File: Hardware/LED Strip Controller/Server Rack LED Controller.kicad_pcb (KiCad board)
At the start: 2 copper layers, 134.6 x 76.2 mm, 168 parts, among them J1 LED_ONE_PWR, J10 UART, J11 CONN_2, J12 LED_THREE_PWR, J13 CONN_3, J14 LED_FOUR_PWR, J15 Conn_01x06_Male, J16 CONN_4, J17 TST, J18 Conn_01x02_Female, J19 Conn_02x04_Odd_Even, J2 Screw_Terminal_01x02, J20 Conn_02x04_Odd_Even, J21 Conn_01x02_Female, J22 Screw_Terminal_01x02, J3 PWR_SWITCH, J4 Conn_02x03_Odd_Even, J5 Conn_01x03_Female, J6 CONN_1, J7 LED_TWO_PWR, J8 SWD, J9 USB_B_Micro, Q1 IRF510N, Q10 IRF510N, Q11 IRF510N, Q12 IRF510N, Q13 IRF510N, Q14 IRF510N, Q15 Q_PMOS_SDG, Q2 IRF510N, Q3 Q_PMOS_SDG, Q4 IRF510N, Q5 IRF510N, Q6 IRF510N, Q7 IRF510N, Q8 IRF510N, Q9 IRF510N, SW1 SW_Push_Dual, U1 STM32F103C8Tx, U2 LM2596S-5, U3 LD1117S50TR_SOT223, U4 LD39050PU33R, U5 INA169, U6 USBLC6-2SC6

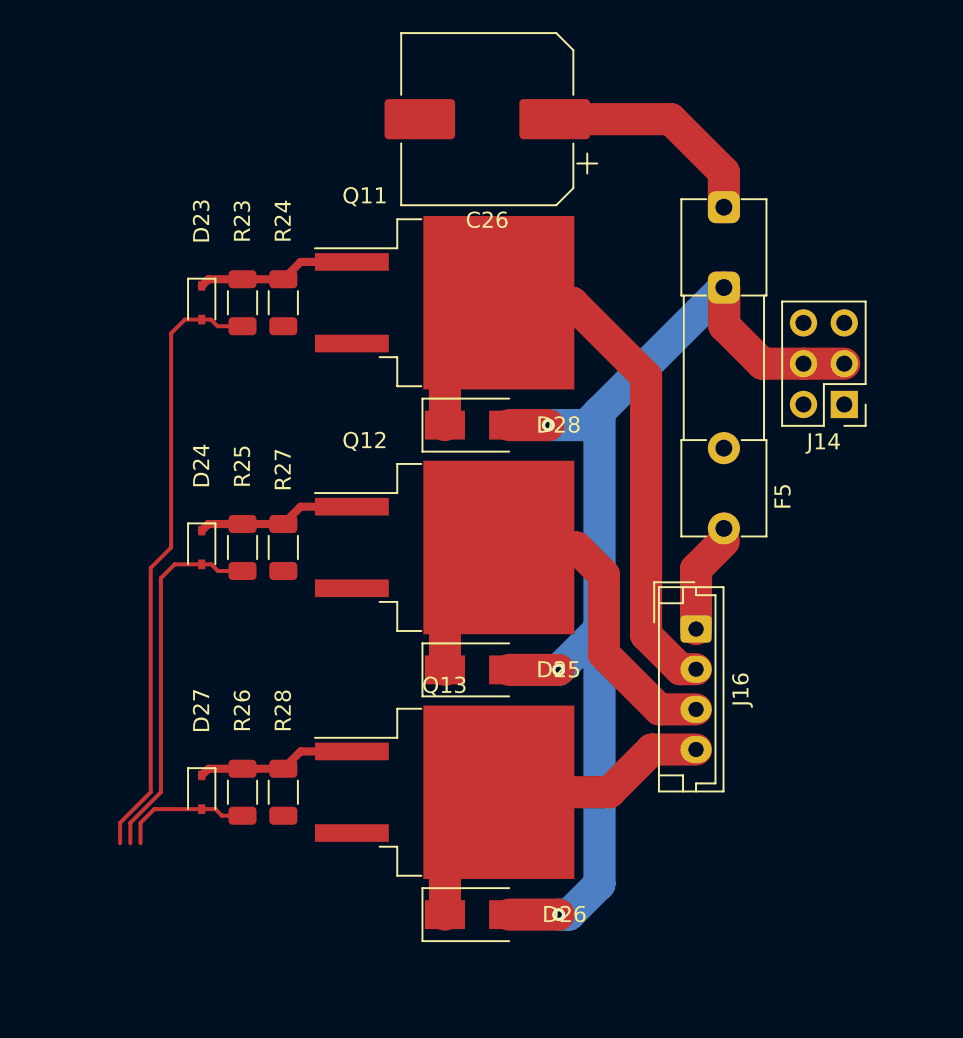
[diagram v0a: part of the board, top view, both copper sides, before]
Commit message: Adding documentation regarding C# User Interface design
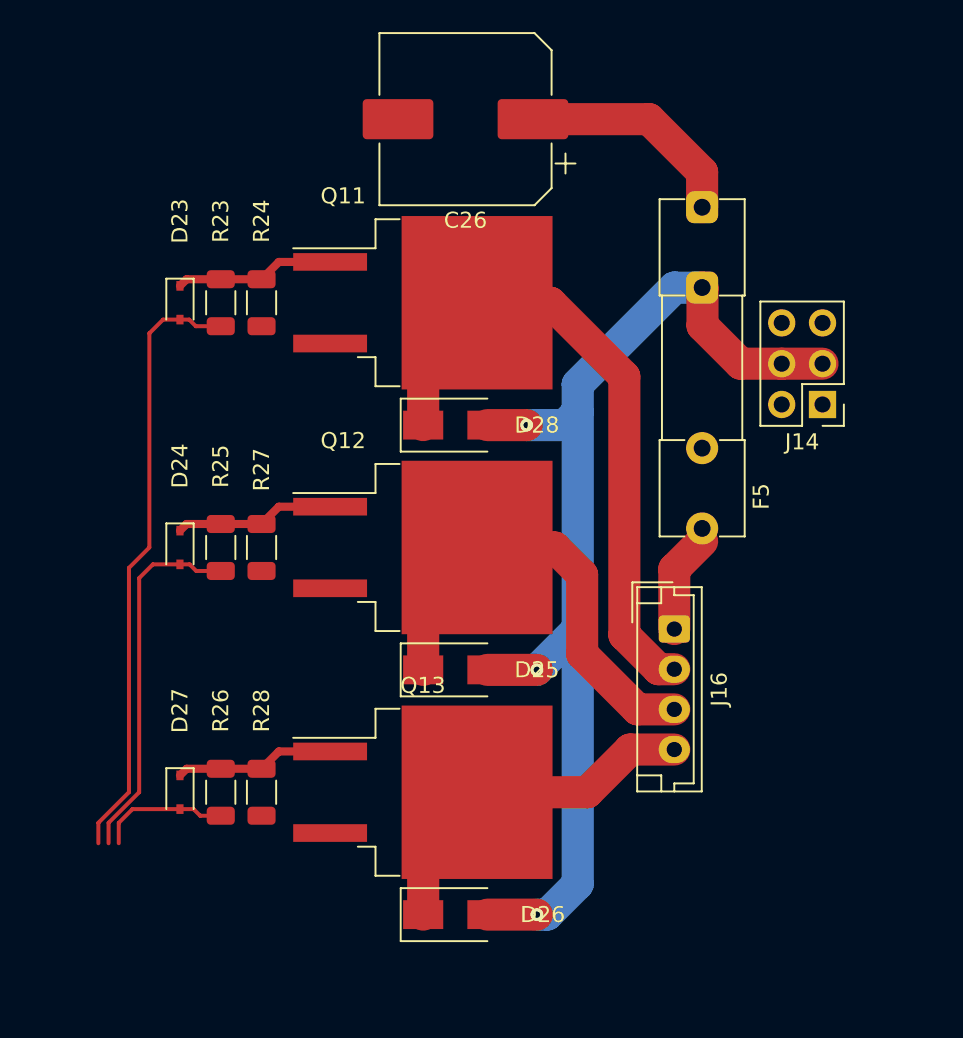
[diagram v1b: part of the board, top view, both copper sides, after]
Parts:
- moved C26 1.36 mm to (69.8, -194.3)
- moved D23 1.36 mm to (52.0, -182.9)
- moved D24 1.36 mm to (52.0, -167.6)
- moved D25 1.36 mm to (69.1, -160.0)
- moved D26 1.36 mm to (69.1, -144.8)
- moved D27 1.36 mm to (52.0, -152.4)
- moved D28 1.36 mm to (69.1, -175.3)
- moved F5 1.36 mm to (84.5, -188.8)
- moved J16 1.36 mm to (82.8, -162.6)
- moved Q11 1.36 mm to (67.1, -182.9)
- moved Q12 1.36 mm to (67.1, -167.6)
- moved Q13 1.36 mm to (67.1, -152.4)
- moved R23 1.36 mm to (54.5, -182.9)
- moved R24 1.36 mm to (57.1, -182.9)
- moved R25 1.36 mm to (54.5, -167.6)
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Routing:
- net CONN_4_5V: track 84.3 -> 85.3 mm
